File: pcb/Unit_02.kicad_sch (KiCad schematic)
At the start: 393 parts, among them J1 AVR-ISP-6, J2 SSD1306, SW1 X1, SW10 F24, SW100 F, SW101 V, SW102 B, SW103 K, SW104 L, SW105 .>, SW106 RMOD2, SW107 RSHIFT, SW108 UPLEFT, SW109 RIGHT, SW11 X2, SW110 KP1, SW111 KP2, SW112 KP3, SW113 LMOD2, SW114 LMOD3, SW115 X, SW116 C, SW117 SPACE, SW118 N, SW119 M, SW12 X3, SW120 ,<, SW121 RMOD1, SW122 RMOD3, SW123 RMOD4, SW124 LEFT, SW125 DOWN, SW126 KP0, SW127 KPDEL, SW128 KPENTER, SW129 RESET, SW13 X4, SW14 X5, SW15 X6, SW16 X7, SW17 ESC, SW18 F13, SW19 F3, SW2 F14, SW20 F4, SW21 F17, SW22 F7, SW23 F8, SW24 F21, SW25 F11, SW26 F12, SW27 Y1, SW28 PRSC, SW29 SCRLK, SW3 F15, SW30 PAUSE, SW31 Y2, SW32 Y3, SW33 `~, SW34 F1, SW35 F2, SW36 4, SW37 F5, SW38 F6, SW39 8, SW4 F16, SW40 F9, SW41 F10, SW42 -_, SW43 =+, SW44 BKSP, SW45 HOME, SW46 PGUP, SW47 KP/, SW48 KP*, SW49 TAB, SW5 F18, SW50 1, SW51 2, SW52 3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

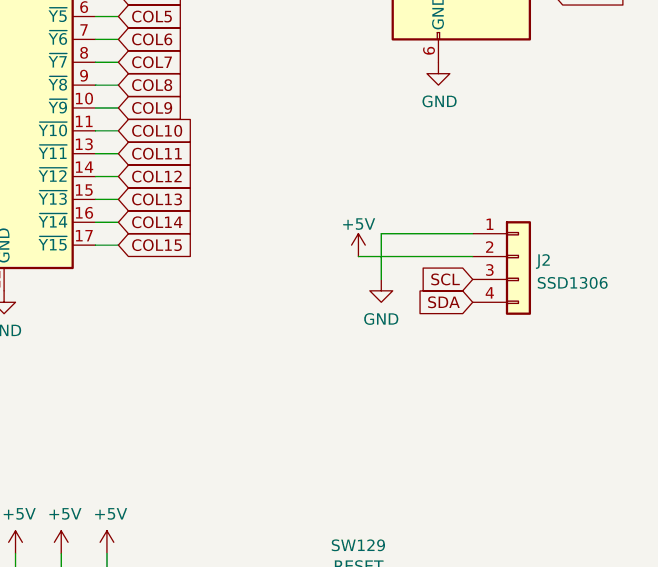
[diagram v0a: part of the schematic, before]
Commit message: Fix PCB errors from v1
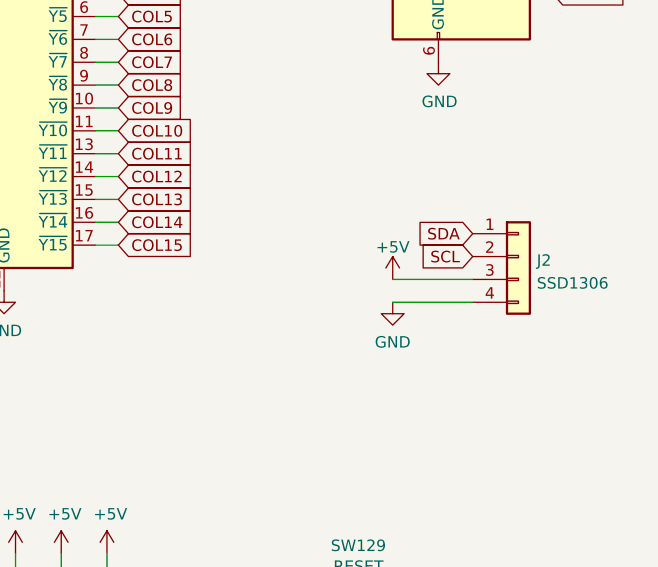
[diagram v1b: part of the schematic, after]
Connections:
- net +5V: now also J2.3 (Pin_3); no longer J2.2 (Pin_2)
- net GND: now also J2.4 (Pin_4); no longer J2.1 (Pin_1)
- net SCL: now also J2.2 (Pin_2); no longer J2.3 (Pin_3)
- net SDA: now also J2.1 (Pin_1); no longer J2.4 (Pin_4)
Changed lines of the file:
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@@
     (stroke (width 0) (type default) (color 0 0 0 0))
   )
+  (wire (pts (xy 355.6 148.59) (xy 364.49 148.59))
+    (stroke (width 0) (type default) (color 0 0 0 0))
+  )
   (wire (pts (xy 63.5 76.2) (xy 63.5 78.74))
     (stroke (width 0) (type default) (color 0 0 0 0))
@@
     (stroke (width 0) (type default) (color 0 0 0 0))
   )
+  (wire (pts (xy 355.6 146.05) (xy 364.49 146.05))
+    (stroke (width 0) (type default) (color 0 0 0 0))
+  )
   (wire (pts (xy 228.6 101.6) (xy 228.6 104.14))
     (stroke (width 0) (type default) (color 0 0 0 0))
@@
     (stroke (width 0) (type default) (color 0 0 0 0))
   )
-  (wire (pts (xy 354.33 140.97) (xy 364.49 140.97))
-    (stroke (width 0) (type default) (color 0 0 0 0))
-  )
   (wire (pts (xy 99.06 96.52) (xy 99.06 109.22))
     (stroke (width 0) (type default) (color 0 0 0 0))
@@
     (stroke (width 0) (type default) (color 0 0 0 0))
   )
-  (wire (pts (xy 351.79 143.51) (xy 364.49 143.51))
-    (stroke (width 0) (type default) (color 0 0 0 0))
-  )
   (wire (pts (xy 50.8 38.1) (xy 50.8 40.64))
     (stroke (width 0) (type default) (color 0 0 0 0))
@@
     (stroke (width 0) (type default) (color 0 0 0 0))
   )
-  (wire (pts (xy 354.33 146.05) (xy 354.33 140.97))
-    (stroke (width 0) (type default) (color 0 0 0 0))
-  )
   (wire (pts (xy 38.1 198.12) (xy 31.75 198.12))
     (stroke (width 0) (type default) (color 0 0 0 0))
@@
     )
   )
-  (global_label "SDA" (shape input) (at 364.49 148.59 180) (fields_autoplaced)
+  (global_label "SDA" (shape input) (at 364.49 140.97 180) (fields_autoplaced)
     (effects (font (size 1.27 1.27)) (justify right))
-    (property "Intersheet References" "${INTERSHEET_REFS}" (id 0) (at 358.5088 148.5106 0)
+    (property "Intersheet References" "${INTERSHEET_REFS}" (id 0) (at 358.5088 140.8906 0)
       (effects (font (size 1.27 1.27)) (justify right) hide)
     )
@@
     )
   )
-  (global_label "SCL" (shape input) (at 364.49 146.05 180) (fields_autoplaced)
+  (global_label "SCL" (shape input) (at 364.49 143.51 180) (fields_autoplaced)
     (effects (font (size 1.27 1.27)) (justify right))
-    (property "Intersheet References" "${INTERSHEET_REFS}" (id 0) (at 358.5693 145.9706 0)
+    (property "Intersheet References" "${INTERSHEET_REFS}" (id 0) (at 358.5693 143.4306 0)
       (effects (font (size 1.27 1.27)) (justify right) hide)
     )
@@
     (pin "4")
   )
-  (symbol (lib_id "power:GND") (at 354.33 146.05 0) (unit 1)
+  (symbol (lib_id "power:GND") (at 355.6 148.59 0) (unit 1)
     (in_bom yes) (on_board yes) (fields_autoplaced)
-    (property "Reference" "#PWR02" (id 0) (at 354.33 152.4 0)
+    (property "Reference" "#PWR02" (id 0) (at 355.6 154.94 0)
       (effects (font (size 1.27 1.27)) hide)
     )
-    (property "Value" "GND" (id 1) (at 354.33 150.4934 0))
-    (property "Footprint" "" (id 2) (at 354.33 146.05 0)
+    (property "Value" "GND" (id 1) (at 355.6 153.0334 0))
+    (property "Footprint" "" (id 2) (at 355.6 148.59 0)
       (effects (font (size 1.27 1.27)) hide)
     )
-    (property "Datasheet" "" (id 3) (at 354.33 146.05 0)
+    (property "Datasheet" "" (id 3) (at 355.6 148.59 0)
       (effects (font (size 1.27 1.27)) hide)
     )
@@
     (pin "4")
   )
-  (symbol (lib_id "power:+5V") (at 351.79 143.51 0) (unit 1)
+  (symbol (lib_id "power:+5V") (at 355.6 146.05 0) (unit 1)
     (in_bom yes) (on_board yes)
-    (property "Reference" "#PWR01" (id 0) (at 351.79 147.32 0)
+    (property "Reference" "#PWR01" (id 0) (at 355.6 149.86 0)
       (effects (font (size 1.27 1.27)) hide)
     )
-    (property "Value" "+5V" (id 1) (at 351.79 139.9342 0))
-    (property "Footprint" "" (id 2) (at 351.79 143.51 0)
+    (property "Value" "+5V" (id 1) (at 355.6 142.4742 0))
+    (property "Footprint" "" (id 2) (at 355.6 146.05 0)
       (effects (font (size 1.27 1.27)) hide)
     )
-    (property "Datasheet" "" (id 3) (at 351.79 143.51 0)
+    (property "Datasheet" "" (id 3) (at 355.6 146.05 0)
       (effects (font (size 1.27 1.27)) hide)
     )
